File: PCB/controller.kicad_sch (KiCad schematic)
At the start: 12 parts, among them J1 DC_Air_Pump, J2 ESP32_Joystick_Module, Q2 IRLZ44N, SW1 SW_SPST, U1 LM2596S-5, U3 ESP32-DEVKITC-32D, U4 MPX5010DP

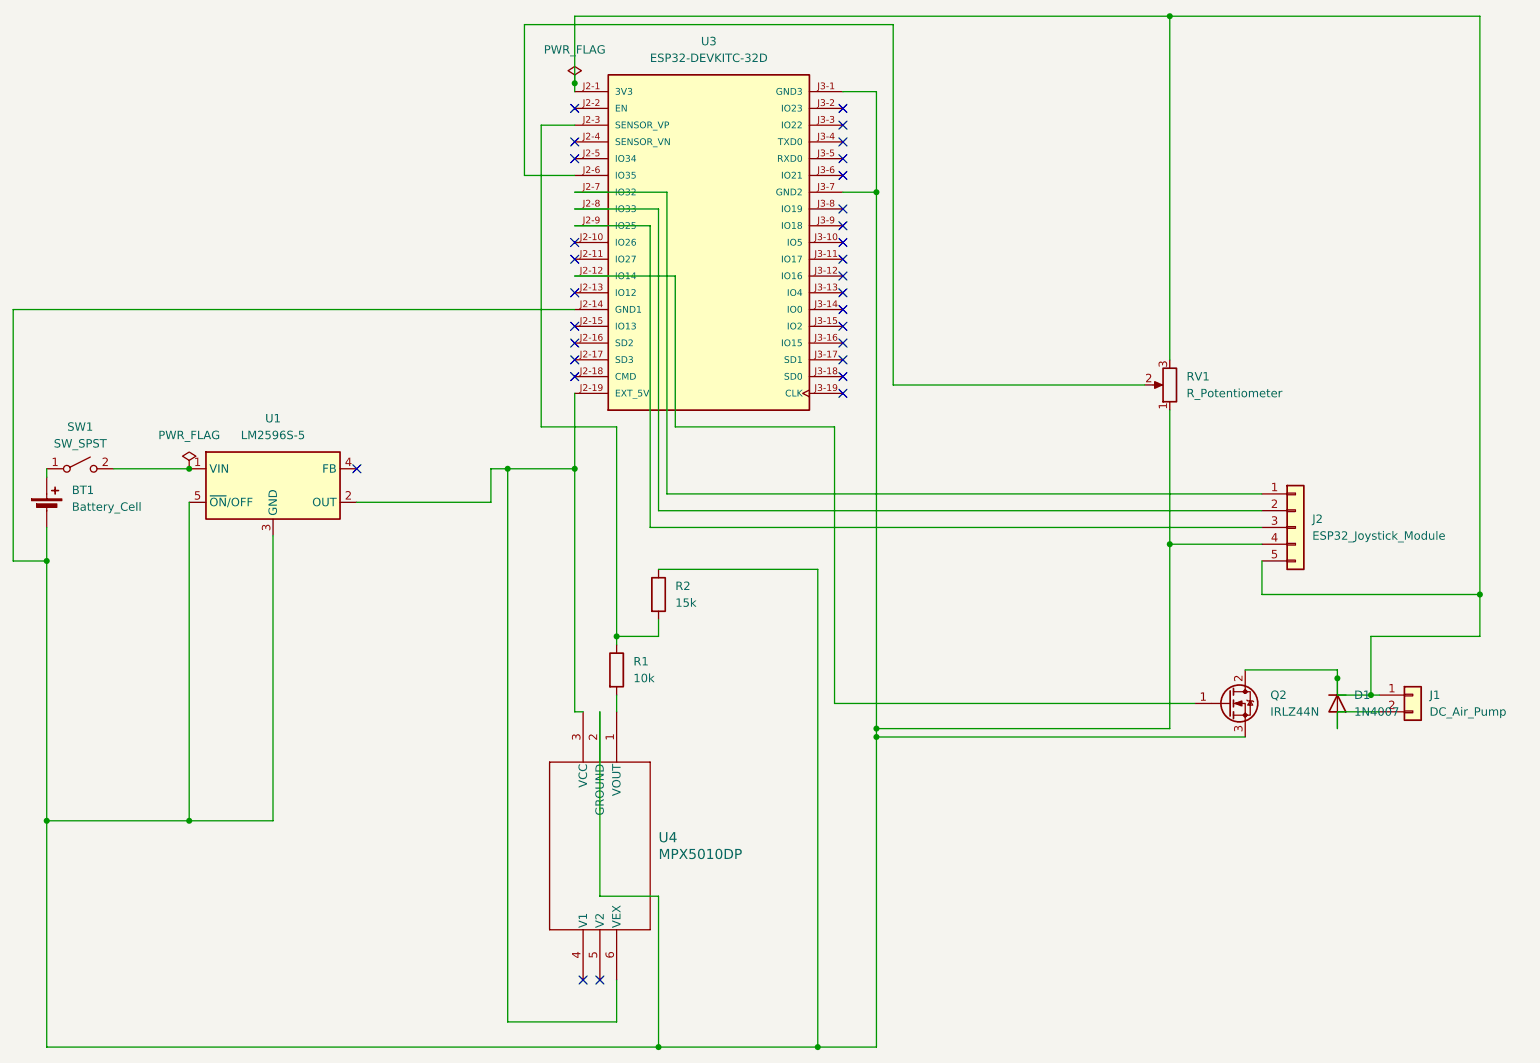
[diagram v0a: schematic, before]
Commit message: Updated PCB and Production Folders (July 6)
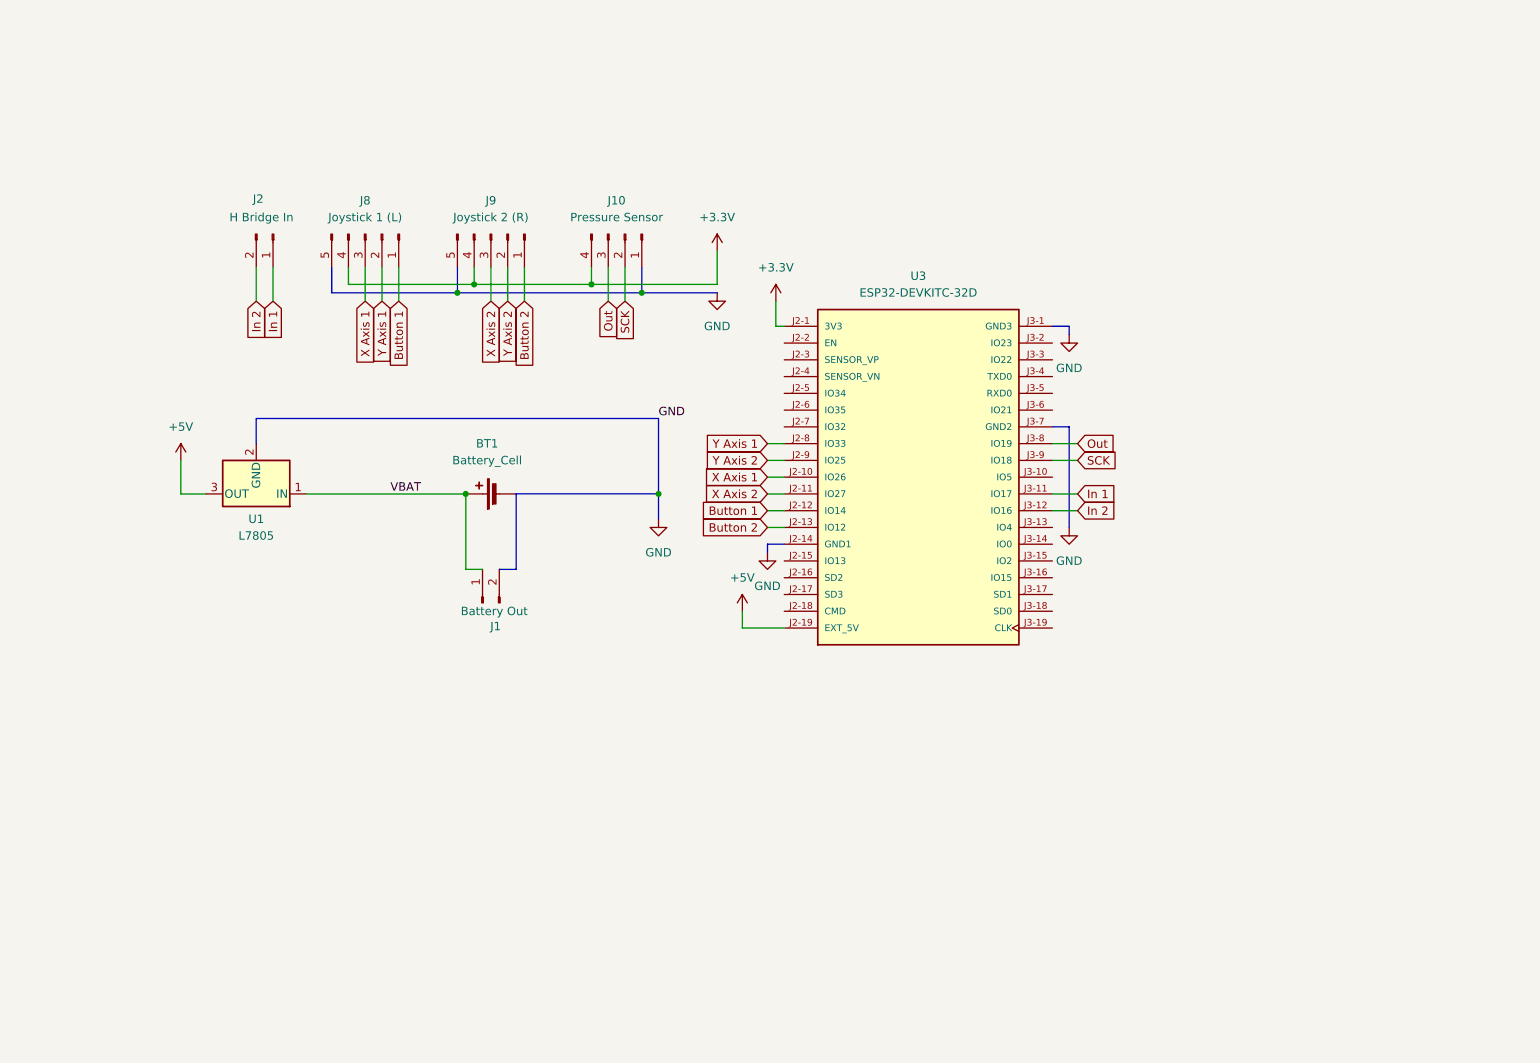
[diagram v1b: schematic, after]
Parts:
- removed D1: 1N4007, Diode_THT:D_DO-41_SOD81_P10.16mm_Horizontal, symbol Diode:1N4007
- removed J1: DC_Air_Pump, TerminalBlock_Phoenix:TerminalBlock_Phoenix_MPT-0,5-3-2.54_1x03_P2.54mm_Horizontal, symbol Connector_Generic:Conn_01x02
- removed J2: ESP32_Joystick_Module, Connector_PinHeader_2.00mm:PinHeader_1x05_P2.00mm_Vertical, symbol Connector_Generic:Conn_01x05
- removed Q2: IRLZ44N, Package_TO_SOT_THT:TO-220-3_Vertical, symbol Transistor_FET:IRLZ44N
- removed R1: 10k, Resistor_THT:R_Axial_DIN0207_L6.3mm_D2.5mm_P7.62mm_Horizontal, symbol Device:R
- removed R2: 15k, Resistor_THT:R_Axial_DIN0207_L6.3mm_D2.5mm_P7.62mm_Horizontal, symbol Device:R
- removed RV1: R_Potentiometer, Potentiometer_THT:Potentiometer_Alps_RK09K_Single_Horizontal, symbol Device:R_Potentiometer
- removed SW1: SW_SPST, Button_Switch_THT:SW_Push_2P1T_Toggle_CK_PVA1xxH1xxxxxxV2, symbol Switch:SW_SPST
- removed U1: LM2596S-5, Package_TO_SOT_SMD:TO-263-5_TabPin3, symbol Regulator_Switching:LM2596S-5
- removed U4: MPX5010DP, controller:MPX5010DP_MOT, symbol controller:MPX5010DP
- added J1: Battery Out, Controller:Battery Connector, symbol Connector:Conn_01x02_Pin
- added J10: Pressure Sensor, Connector_PinHeader_2.54mm:PinHeader_1x04_P2.54mm_Vertical, symbol Connector:Conn_01x04_Pin
- added J2: H Bridge In, Connector_PinHeader_2.54mm:PinHeader_1x02_P2.54mm_Vertical, symbol Connector:Conn_01x02_Pin
- added J8: Joystick 1 (L), Connector_PinHeader_2.54mm:PinHeader_1x05_P2.54mm_Vertical, symbol Connector:Conn_01x05_Pin
- added J9: Joystick 2 (R), Connector_PinHeader_2.54mm:PinHeader_1x05_P2.54mm_Vertical, symbol Connector:Conn_01x05_Pin
- added U1: L7805, Package_TO_SOT_THT:TO-220-3_Vertical, symbol Regulator_Linear:L7805
- BT1: footprint Connector_JST:JST_PH_S2B-PH-K_1x02_P2.00mm_Horizontal -> Controller:Battery Connector
- U3: footprint ESP32_controller:MODULE_ESP32-DEVKITC-32D -> Controller:ESP32
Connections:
- net Y Axis 1: now reaches U3.J2-8 (IO33)
- net Y Axis 1: now also J8.2 (Pin_2)
- net Y Axis 2: now reaches U3.J2-9 (IO25)
- net Y Axis 2: now also J9.2 (Pin_2)
- net +3.3V: now reaches U3.J2-1 (3V3)
- net +3.3V: now also J10.4 (Pin_4), J8.4 (Pin_4), J9.4 (Pin_4)
- net VBAT: now reaches BT1.1 (+)
- net VBAT: now also J1.1 (Pin_1), U1.1 (IN)
- net Button 1: now reaches U3.J2-12 (IO14)
- net Button 1: now also J8.1 (Pin_1)
- net X Axis 1: now reaches U3.J2-10 (IO26)
- net X Axis 1: now also J8.3 (Pin_3)
- net X Axis 2: now reaches U3.J2-11 (IO27)
- net X Axis 2: now also J9.3 (Pin_3)
- net Button 2: now reaches U3.J2-13 (IO12)
- net Button 2: now also J9.1 (Pin_1)
- net +5V: now reaches U3.J2-19 (EXT_5V)
- net +5V: now also U1.3 (OUT)
- net In 1: now reaches U3.J3-11 (IO17)
- net In 1: now also J2.1 (Pin_1)
- net In 2: now reaches U3.J3-12 (IO16)
- net In 2: now also J2.2 (Pin_2)
- net Out: now reaches U3.J3-8 (IO19)
- net Out: now also J10.3 (Pin_3)
- net SCK: now reaches U3.J3-9 (IO18)
- net SCK: now also J10.2 (Pin_2)
- now unconnected: BT1.2 (-), U3.J2-14 (GND1), U3.J3-1 (GND3), U3.J3-7 (GND2)
- no-connect marks 30 -> 0
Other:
- moved on the sheet: U3
